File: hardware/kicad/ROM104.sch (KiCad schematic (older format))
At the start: 41 parts, among them J1 Screw_Terminal_01x06, J2 Screw_Terminal_01x06, J3 Screw_Terminal_01x06, J4 CAN, K1 SPDT_RELAY, K2 SPDT_RELAY, K3 SPDT_RELAY, K4 SPDT_RELAY, K5 SPDT_RELAY, K6 SPDT_RELAY, SW1 INSTANCE, SW2 BUS, SW3 PRG, U1 L293D, U2 L293D, U3 74HC595, U4 L293D, U5 MCP2551-I-P, U6 TMR_2411, U7 Teensy_3.2

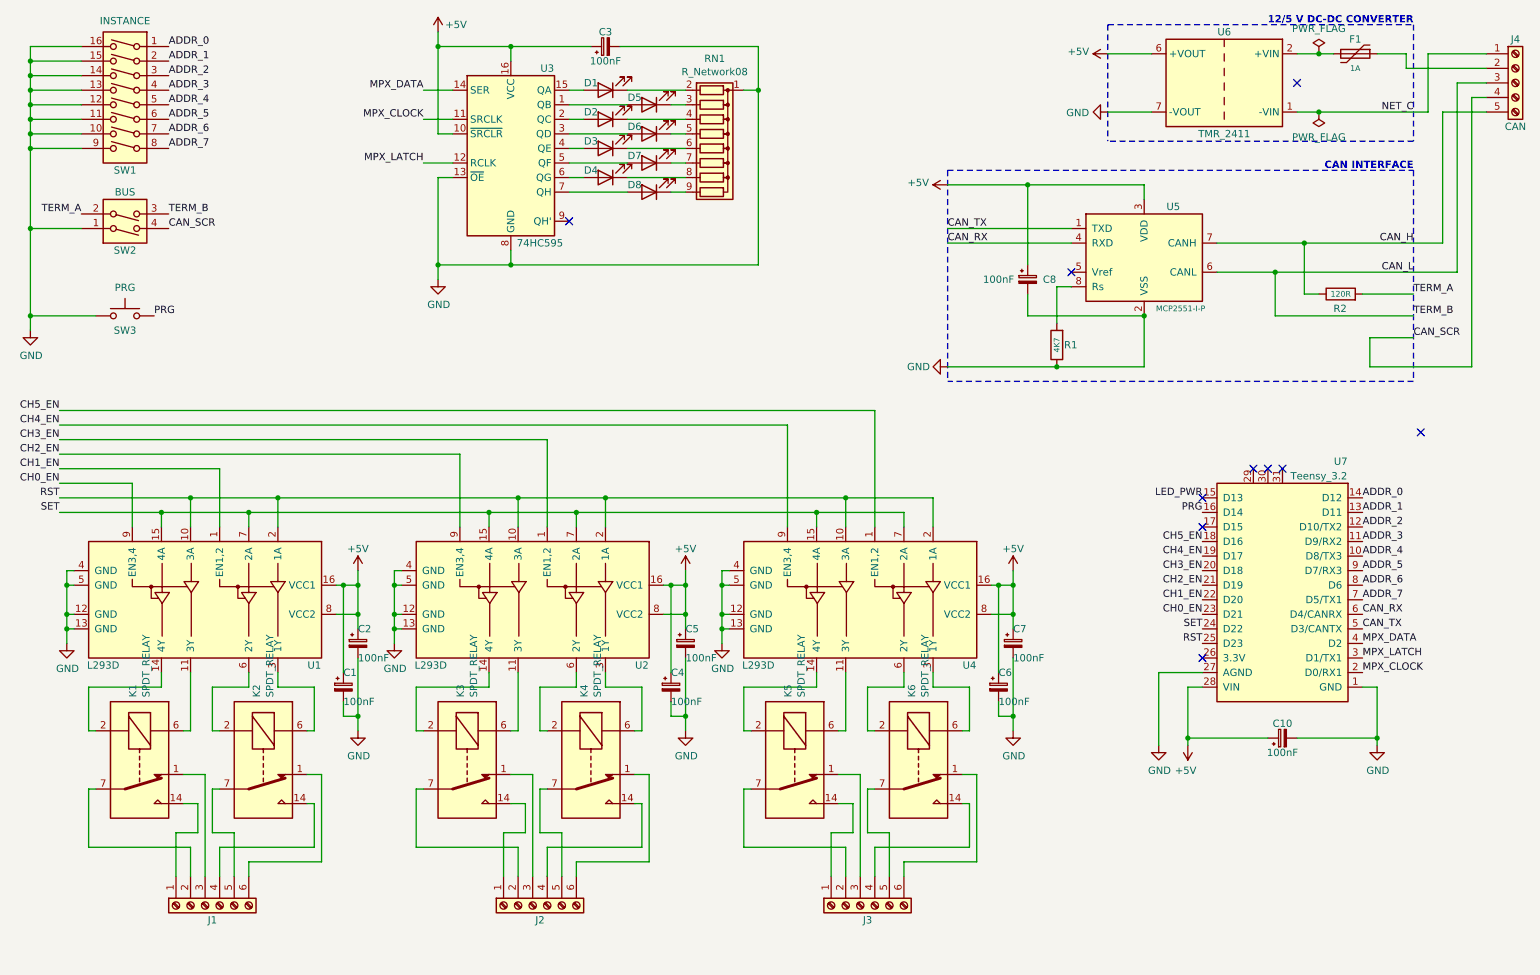
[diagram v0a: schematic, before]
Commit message: PCB update
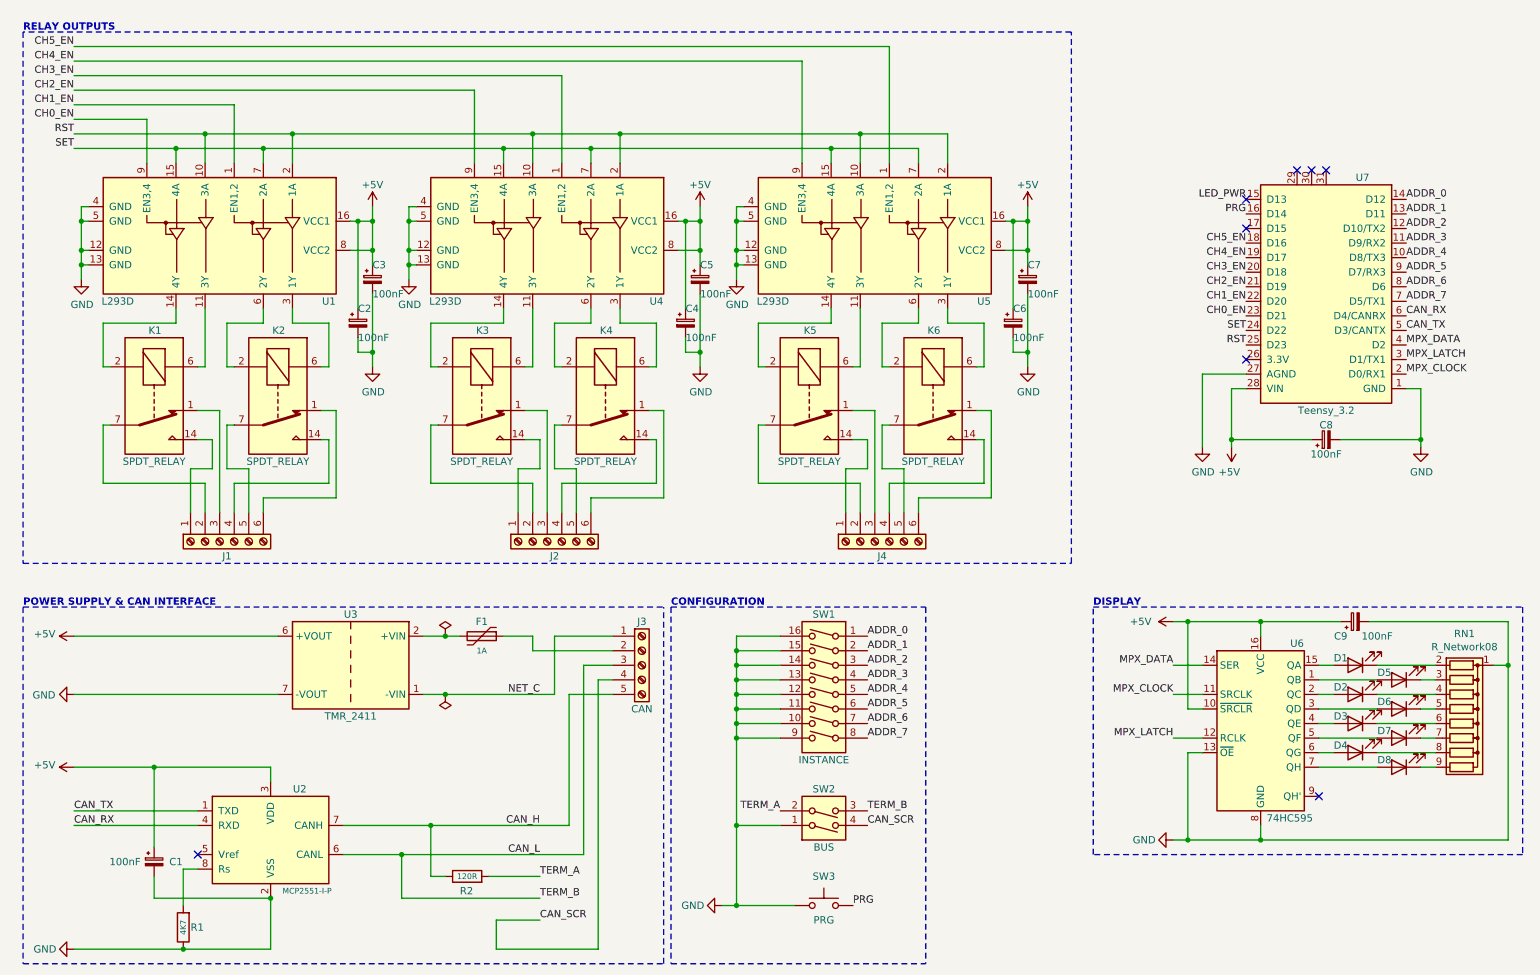
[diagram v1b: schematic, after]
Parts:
- SW3: footprint Button_Switch_THT:SW_PUSH_6mm -> PDJR-connectors:PCB_PUSH_BUTTON
- renumbered C8 to C1, C1 to C2, C2 to C3, C10 to C8, C3 to C9, J4 to J3, J3 to J4, U5 to U2, U6 to U3, U2 to U4, U4 to U5, U3 to U6
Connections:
- no-connect marks 10 -> 8
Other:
- note added: "CONFIGURATION"
- note added: "DISPLAY"
- note added: "POWER SUPPLY & CAN INTERFACE"
- note added: "RELAY OUTPUTS"
- note removed: "12/5 V DC-DC CONVERTER"
- note removed: "CAN INTERFACE"
- moved on the sheet: C1, C2, C3, C4, C5, C6, C7, C8, C9, D1, D2, D3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
